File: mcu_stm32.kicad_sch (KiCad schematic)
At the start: 1 part, among them U1 STM32F103C6Tx

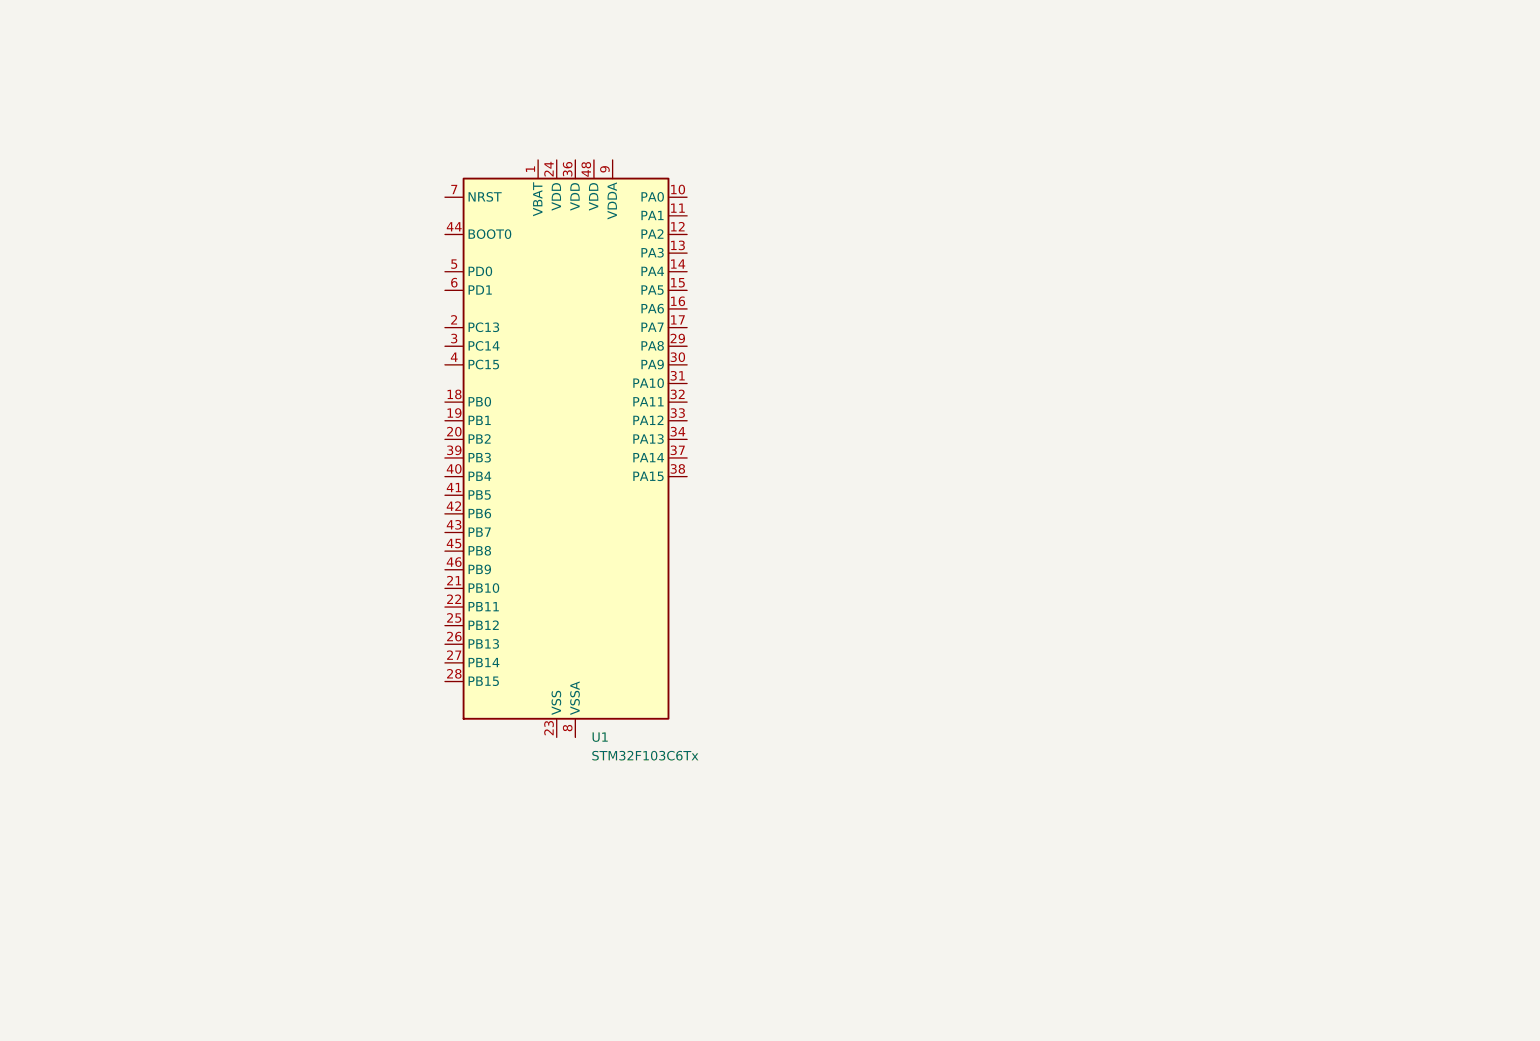
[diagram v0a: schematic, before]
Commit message: stm32 added
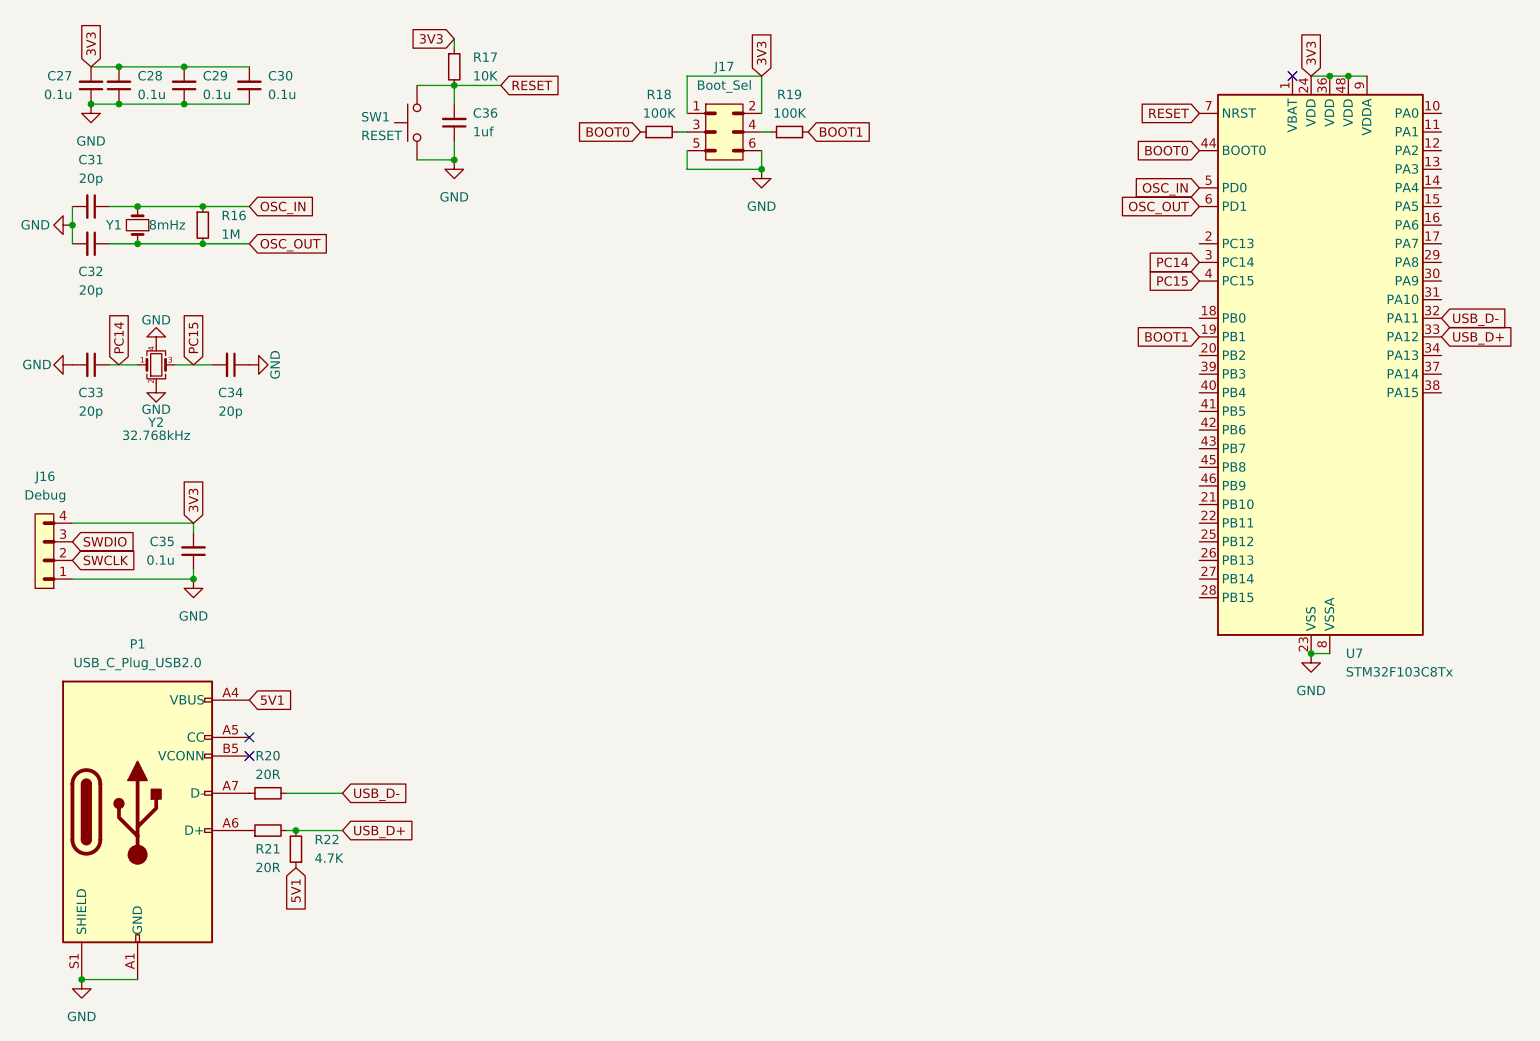
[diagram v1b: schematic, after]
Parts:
- removed U1: STM32F103C6Tx, Package_QFP:LQFP-48_7x7mm_P0.5mm, symbol MCU_ST_STM32F1:STM32F103C6Tx
- added C27, C28, C29, C30, C35: 0.1u, Capacitor_SMD:C_0805_2012Metric, symbol Device:C_Small
- added C31, C32, C33, C34: 20p, Capacitor_SMD:C_0805_2012Metric, symbol Device:C_Small
- added C36: 1uf, Capacitor_SMD:C_0805_2012Metric, symbol Device:C_Small
- added J16: Debug, Connector_PinHeader_2.54mm:PinHeader_1x04_P2.54mm_Vertical, symbol PCM_SL_Pin_Headers:PINHD_1x4_Male
- added J17: Boot_Sel, Connector_PinHeader_2.54mm:PinHeader_2x03_P2.54mm_Vertical, symbol PCM_SL_Pin_Headers:PINHD_2x3_Male
- added P1: USB_C_Plug_USB2.0, symbol Connector:USB_C_Plug_USB2.0
- added R16: 1M, Resistor_SMD:R_0805_2012Metric, symbol Device:R_Small
- added R17: 10K, Resistor_SMD:R_0805_2012Metric, symbol Device:R_Small
- added R18, R19: 100K, Resistor_SMD:R_0805_2012Metric, symbol Device:R_Small
- added R20, R21: 20R, Resistor_SMD:R_0805_2012Metric, symbol Device:R_Small
- added R22: 4.7K, Resistor_SMD:R_0805_2012Metric, symbol Device:R_Small
- added SW1: RESET, Button_Switch_SMD:SW_SPST_CK_KMS2xxGP, symbol Switch:SW_Push
- added U7: STM32F103C8Tx, Package_QFP:LQFP-48_7x7mm_P0.5mm, symbol MCU_ST_STM32F1:STM32F103C8Tx
- added Y1: 8mHz, symbol Device:Crystal_Small
- added Y2: 32.768kHz, symbol Device:Crystal_GND24_Small
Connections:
- new net: J17.3, R18.2
- new net: P1.A6 (D+), R21.1
- new net: J17.4, R19.1
- new net: P1.A7 (D-), R20.1
- new net 3V3: C27.2, C28.2, C29.2, C30.2, C35.2, J16.4, J17.1, J17.2, R17.1, U7.24 (VDD), U7.36 (VDD), U7.48 (VDD), U7.9 (VDDA)
- new net 5V1: P1.A4 (VBUS), P1.A9 (VBUS), P1.B4 (VBUS), P1.B9 (VBUS), R22.1
- new net BOOT0: R18.1, U7.44 (BOOT0)
- new net BOOT1: R19.2, U7.19 (PB1)
- new net GND: C27.1, C28.1, C29.1, C30.1, C31.2, C32.2, C33.2, C34.1, C35.1, C36.1, J16.1, J17.5, J17.6, P1.A1 (GND), P1.A12 (GND), P1.B1 (GND), P1.B12 (GND), P1.S1 (SHIELD), SW1.1, U7.23 (VSS), U7.35 (VSS), U7.47 (VSS), U7.8 (VSSA), Y2.2, Y2.4
- new net OSC_IN: C31.1, R16.1, U7.5 (PD0), Y1.2
- new net OSC_OUT: C32.1, R16.2, U7.6 (PD1), Y1.1
- new net PC14: C33.1, U7.3 (PC14), Y2.1
- new net PC15: C34.2, U7.4 (PC15), Y2.3
- new net RESET: C36.2, R17.2, SW1.2, U7.7 (NRST)
- new net SWCLK: J16.2
- new net SWDIO: J16.3
- new net USB_D+: R21.2, R22.2, U7.33 (PA12)
- new net USB_D-: R20.2, U7.32 (PA11)
- no-connect marks 0 -> 3
